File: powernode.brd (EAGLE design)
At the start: 100 x 50 mm, 35 parts, among them SW1 ROTARTY_ENCODER, U1 LCD-16X2NOHOLES, X1 5566-4, X2 5566-6, X3 5566-24

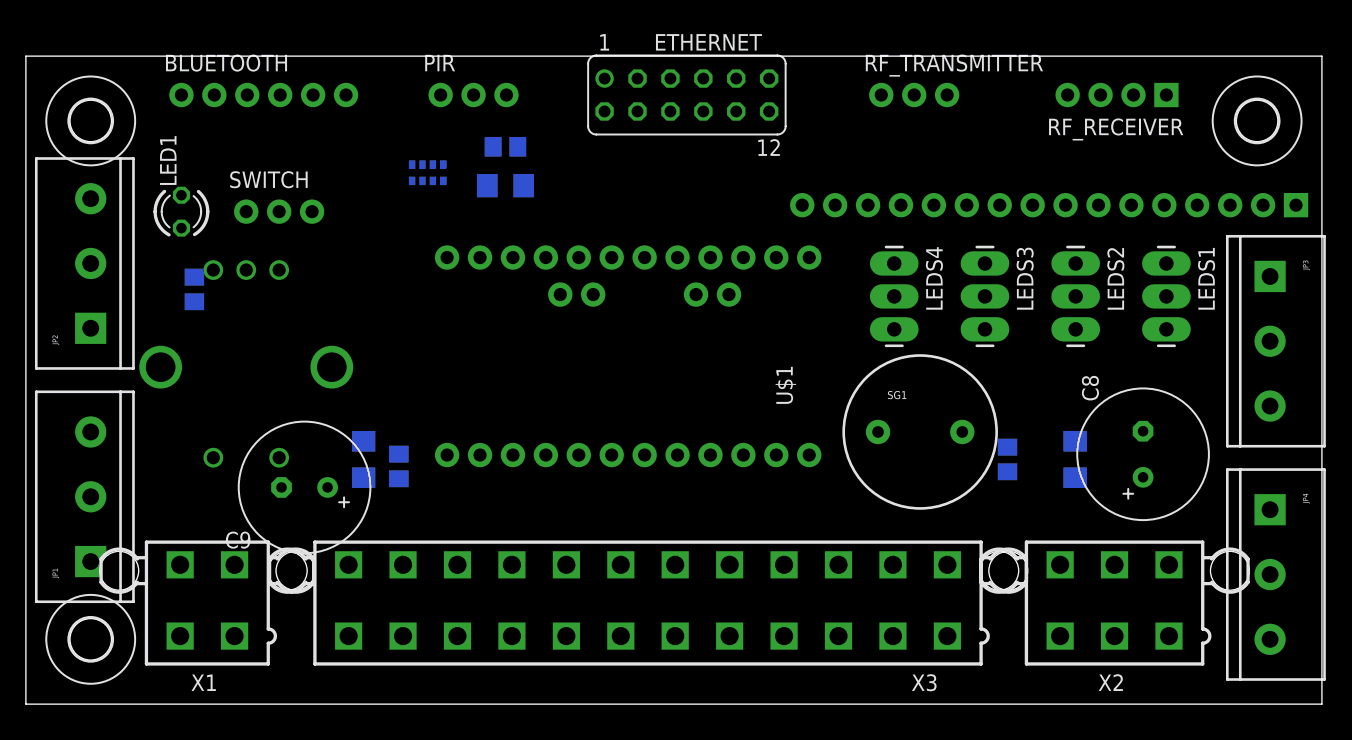
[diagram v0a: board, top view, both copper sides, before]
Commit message: Work on powernode.
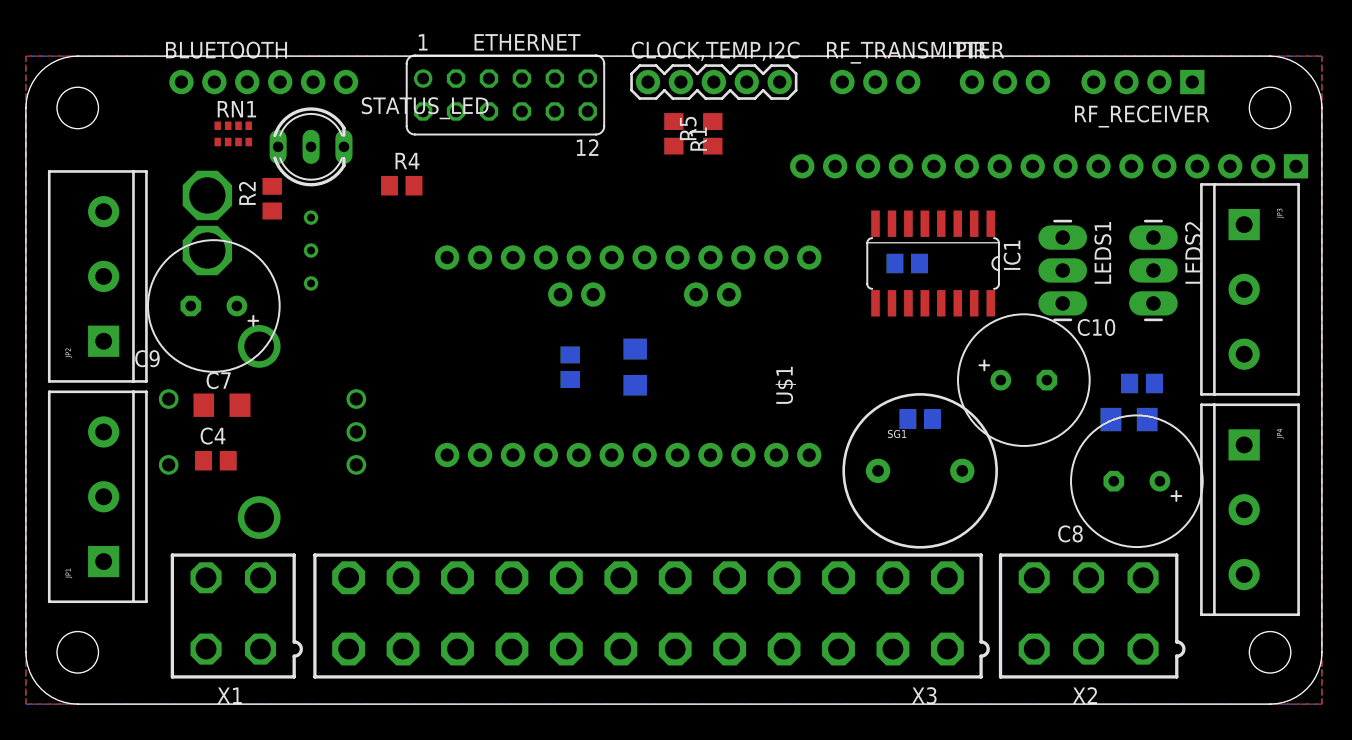
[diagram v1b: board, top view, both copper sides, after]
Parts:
- removed H1, H2, H3: MOUNT-HOLE3.2, holes:3,2
- removed LED1: (no value), led:LED3MM
- removed LEDS3, LEDS4: (no value), SparkFun-Connectors:1X03_LONGPADS
- removed SWITCH: (no value), SparkFun-Connectors:1X03_NO_SILK
- added C10: 100 uF, rcl:E3,5-10
- added C11, C3: 100 nF, rcl:C0805
- added CLOCK,TEMP,I2C: (no value), SparkFun:1X05
- added IC1: 74HC595D, 74xx-eu:SO16
- added POWER_SWITCH: KNC1-101-2P, knc1-101-switch:KNC1-101-2P
- added R2, R4: (no value), rcl:R0805
- added R3: 10k, resistor:RTRIM3296W
- added R5: (4k), rcl:R0805
- added STATUS_LED: (no value), led:DUOLED-C-5MM
- R1: value (none) -> (4k)
- X1: device con-molex:5566-4 -> con-molex--with-atx-connectors-without-side-screws:5566-4
- X2: device con-molex:5566-6 -> con-molex--with-atx-connectors-without-side-screws:5566-6
- X3: device con-molex:5566-24 -> con-molex--with-atx-connectors-without-side-screws:5566-24
- moved PIR 41.0 mm to (73.0, 48.0)
- moved R1 38.9 mm to (50.0, 44.0), flipped to the top
- moved C2 17.7 mm to (42.0, 26.0), turned to 270 degrees
- moved C1 17.2 mm to (47.0, 26.0), turned to 270 degrees
- moved C9 15.7 mm to (14.5, 30.7)
- moved RN1 15.3 mm to (16.0, 44.0), flipped to the top
- moved C4 14.1 mm to (14.7, 18.8), flipped to the top, turned to 0 degrees
- moved ETHERNET 14.0 mm to (37.0, 47.0)
- moved C5 11.9 mm to (86.1, 24.7), turned to 0 degrees
- moved C7 11.7 mm to (15.1, 23.1), flipped to the top, turned to 0 degrees
- moved LEDS1 8.25 mm to (80.0, 36.0)
- moved LEDS2 6.32 mm to (87.0, 36.0)
- moved JP4 5.39 mm to (94.0, 20.0)
- moved C6 5.18 mm to (85.1, 22.0), turned to 0 degrees
- moved SW1 5.10 mm to (18.0, 21.0), turned to 180 degrees
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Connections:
- removed net A: U1.15
- removed net K: U1.16
- removed net LEDSTRIP3: LEDS3.2
- removed net LEDSTRIP4: LEDS4.2
- removed net N$12: U$1.6
- removed net N$13: U$1.7
- removed net N$14: U$1.8
- removed net N$15: U$1.9
- removed net N$16: U$1.10
- removed net N$18: U$1.12
- removed net N$19: U$1.A4
- removed net N$20: U$1.A5
- removed net N$22: U$1.24
- removed net N$6: LED1.A, R1.1
- removed net VDD: U1.2
- removed net VSS: U1.1
- new net BUZZER: C11.2, IC1.15, SG1.-
- new net ERROR_LED: IC1.7, R4.2
- new net LCD_BACKLIGHT: IC1.1, U1.16
- new net LCD_CLOCK: IC1.11, U$1.12
- new net LCD_DATA: IC1.14, U$1.A7
- new net LCD_ENABLE: IC1.12, U$1.13, U1.6
- new net N$7: IC1.4, U1.12
- new net SCL: CLOCK,TEMP,I2C.4, R1.2, U$1.A5
- new net SDA: CLOCK,TEMP,I2C.3, R5.2, U$1.A4
- new net TEMPERATURE_DS: CLOCK,TEMP,I2C.5
- new net TURN_WHEEL_A: SW1.A, U$1.5
- new net TURN_WHEEL_B: SW1.B, U$1.6
- new net TURN_WHEEL_CLICK: SW1.SW+, U$1.7
- net +12V: now also R2.2; no longer LEDS3.1, LEDS4.1, R1.2
- net +5V/2: now also C10.+, C11.1, C3.1, CLOCK,TEMP,I2C.2, IC1.10, IC1.16, R1.1, R3.3, R5.1, SG1.+, U1.15, U1.2; no longer SWITCH.3
- net GND: now also C10.-, C3.2, CLOCK,TEMP,I2C.1, IC1.13, IC1.8, POWER_SWITCH.P$1, R3.1, STATUS_LED.C, SW1.C, SW1.SW-, U1.1, U1.5; no longer LED1.K, LEDS3.3, LEDS4.3, SWITCH.1
- net LEDSTRIP1: now also U$1.9
- net LEDSTRIP2: now also U$1.10
- net N$1: now also IC1.3, U1.11; no longer U$1.A6
- net N$10: now also U1.3; no longer U$1.20
- net N$11: now also R4.1, STATUS_LED.AR; no longer U$1.5
- net N$2: now also IC1.2, U1.4; no longer U$1.A7
- net N$3: now also POWER_SWITCH.P$2, RN1.4; no longer U$1.13
- net N$5: now also R2.1, STATUS_LED.AX; no longer RN1.4, SWITCH.2
- net N$8: now also IC1.5, U1.13; no longer U$1.18
- net N$9: now also IC1.6, U1.14; no longer U$1.19
- net POWER_SWITCH: now also U$1.8
- net PROXIMITY: now also U$1.20
- net PS_ON: now also U$1.A6
- net RF_DATA_IN: now also U$1.18
- net RF_DATA_OUT: now also U$1.19
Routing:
- added copper zone on layer 1, net +12V
- added copper zone on layer 16, net GND
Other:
- outline, holes or cut-outs redrawn
